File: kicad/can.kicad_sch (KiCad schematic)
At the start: 23 parts, among them CN10 KF2EDGR-2.54-3P, J4 Header-Male-2.54_2x2, U18 ADM3057EBRWZ-RL

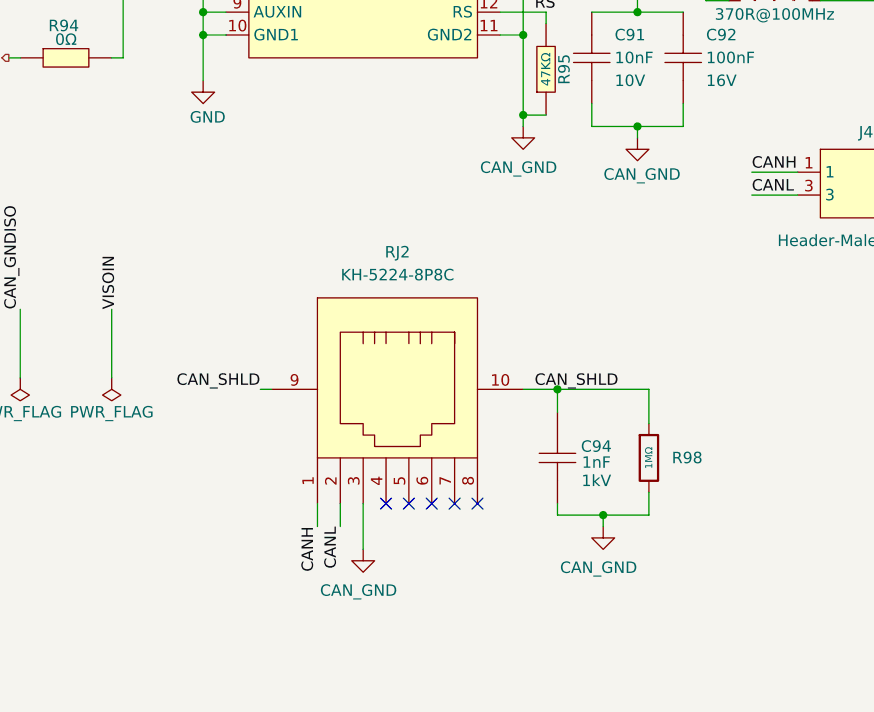
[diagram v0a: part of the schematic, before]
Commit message: Updates
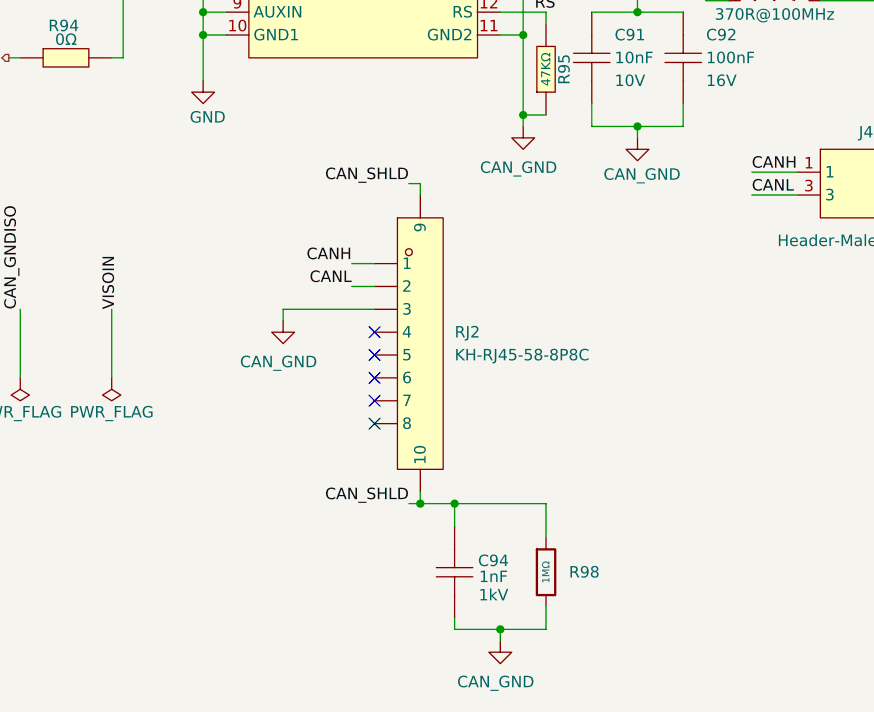
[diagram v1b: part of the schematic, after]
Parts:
- removed RJ2: KH-5224-8P8C, MyParts:RJ45-KH-5224-8P8C, symbol MyParts:KH-5224-8P8C
- added RJ2: KH-RJ45-58-8P8C, MyParts:RJ45-TH_KH-RJ45-58-8P8C, symbol MyParts:KH-RJ45-58-8P8C
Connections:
- net CANH: now also RJ2.1
- net CANL: now also RJ2.2
- net CAN_GND: now also RJ2.3
- net CAN_SHLD: now also RJ2.10, RJ2.9
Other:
- moved on the sheet: C94, R98

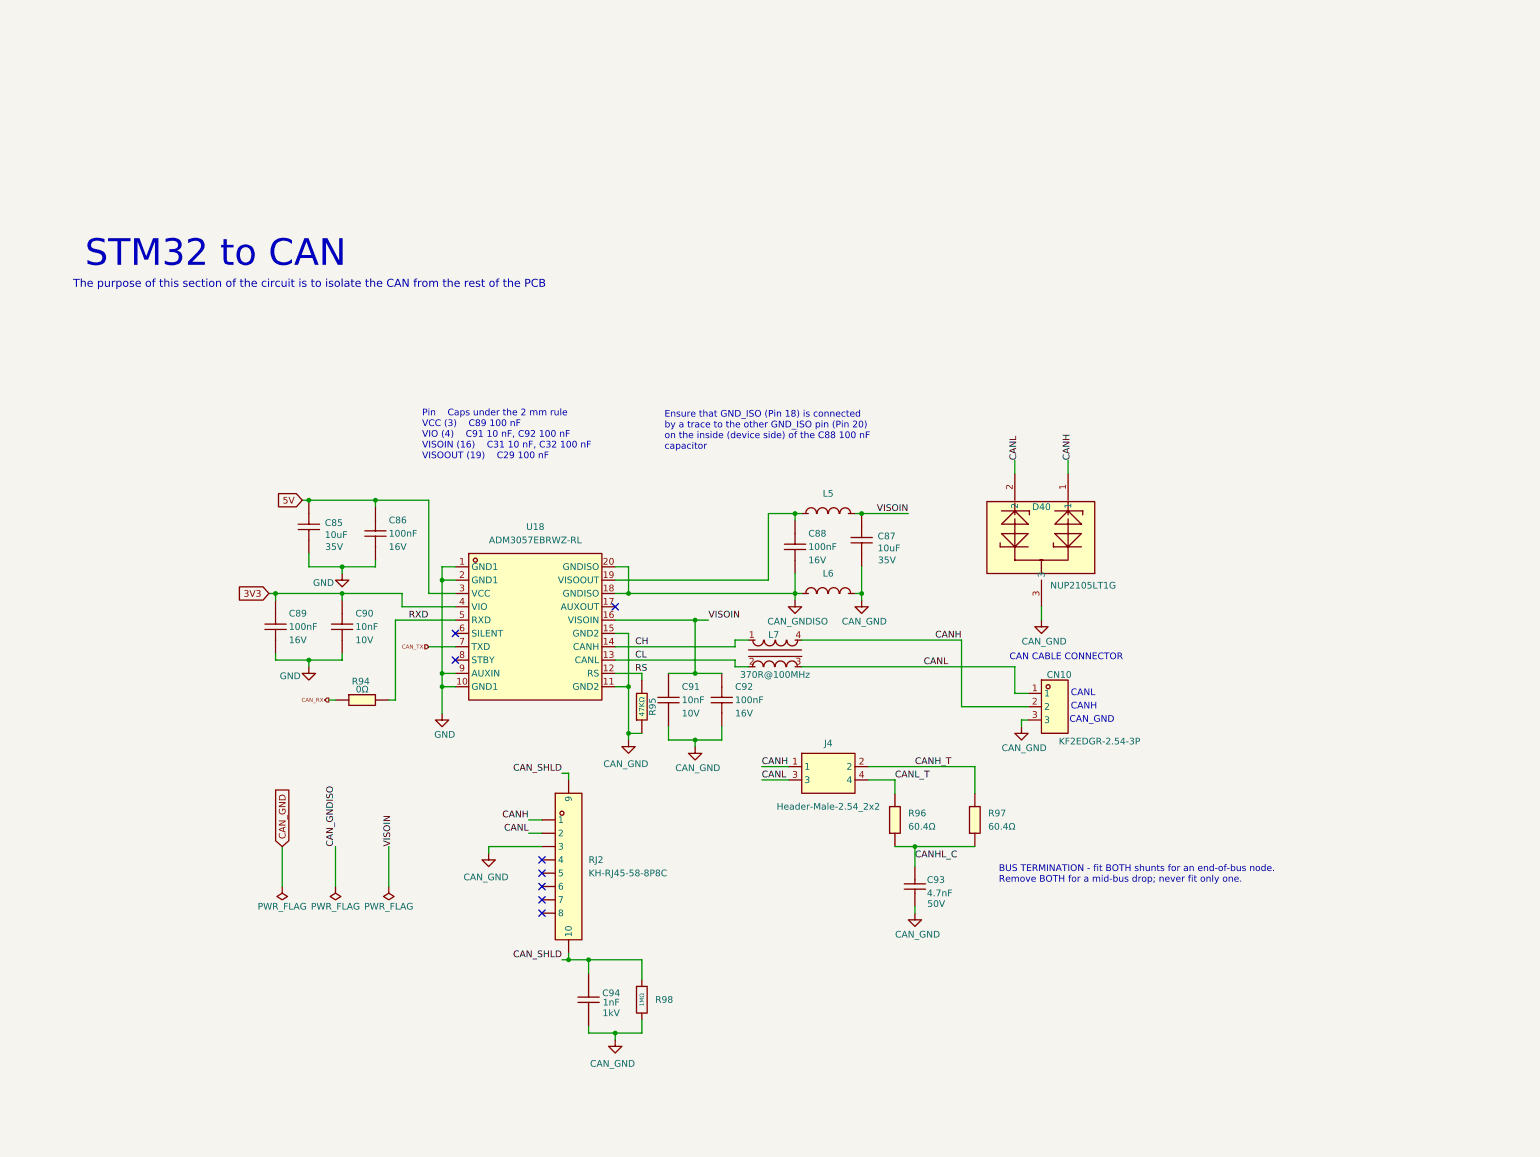
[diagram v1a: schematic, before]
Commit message: Before removing CAN 24V
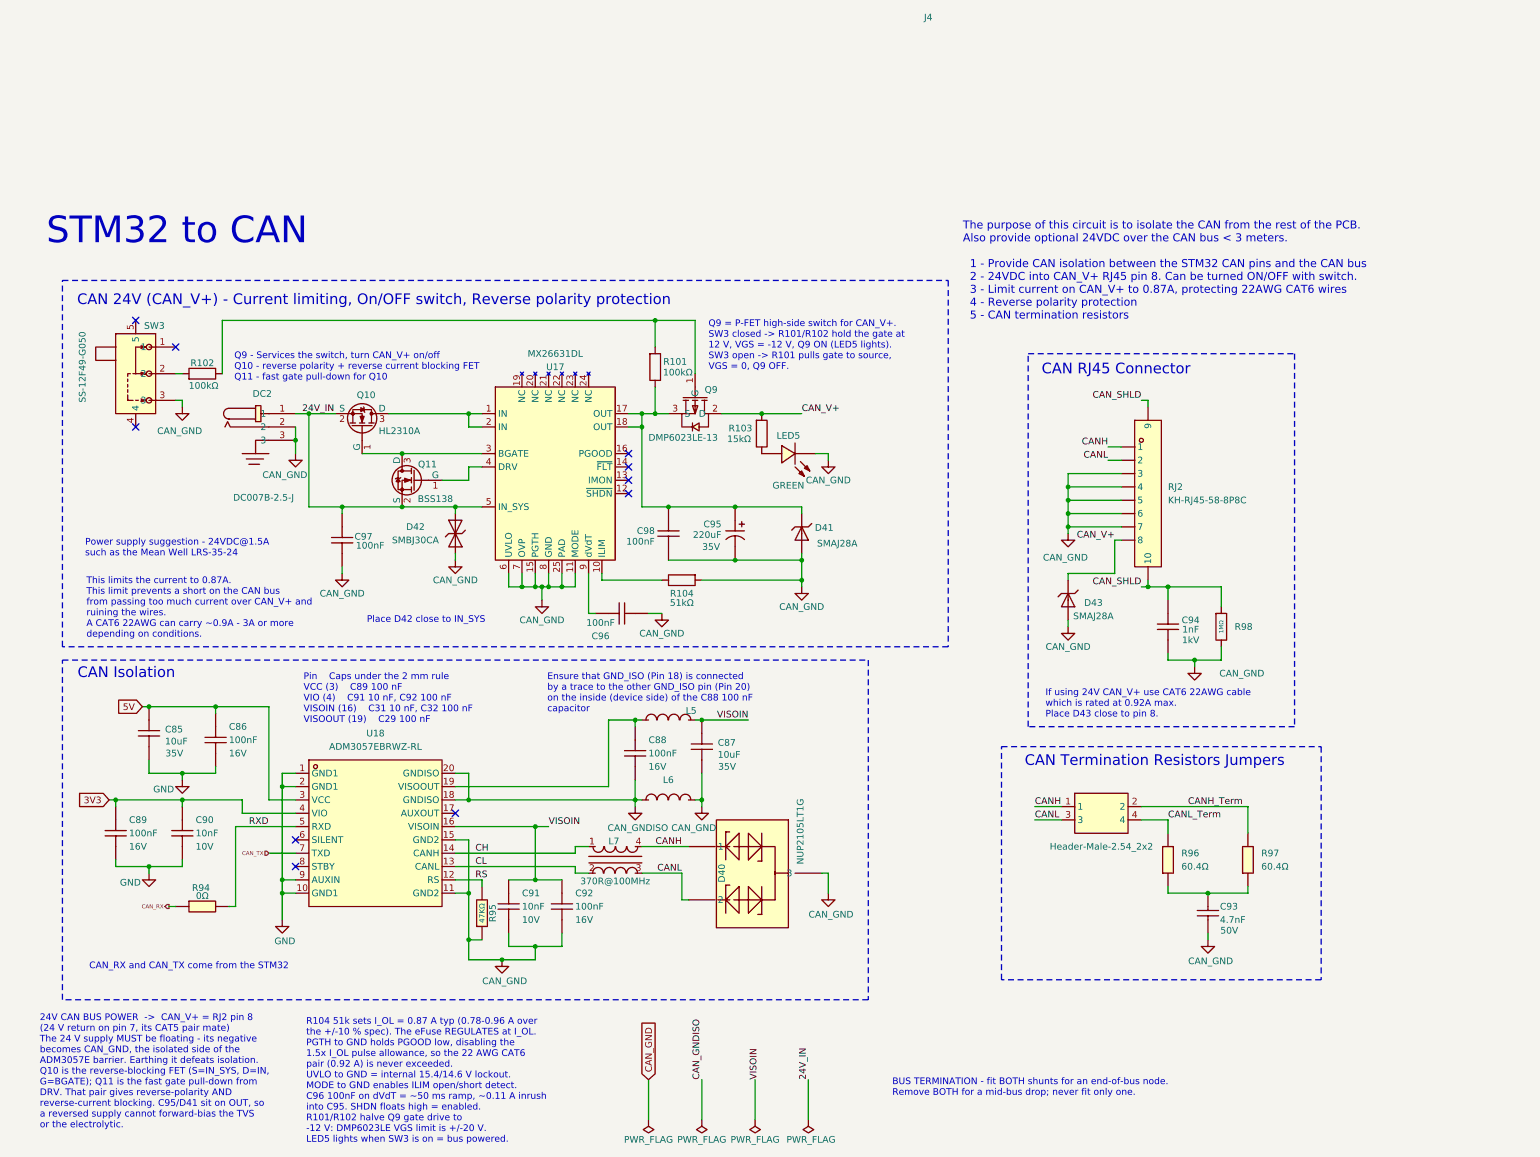
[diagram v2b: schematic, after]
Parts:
- removed CN10: KF2EDGR-2.54-3P, MyParts:CONN-TH_3P-P2.54_KF2EDGR-2.54-3P, symbol MyParts:KF2EDGR-2.54-3P
- added C95: 220uF, MyParts:CAP-SMD_BD6.3-L6.6-W6.6-FD, symbol MyParts:JVJ35V220M6X8
- added C96, C97, C98: 100nF, MyParts:C0402, symbol MyParts:CL05B104KO5NNNC
- added D41, D43: SMAJ28A, PCM_JLCPCB:D_SMA, symbol PCM_JLCPCB-Diodes:TVS-Uni,SMAJ28A
- added D42: SMBJ30CA, PCM_JLCPCB:D_SMB, symbol PCM_JLCPCB-Diodes:TVS-Bi,SMBJ30CA
- added DC2: DC007B-2.5-J, MyParts:DC-IN-TH_HX-DC007B-2.5, symbol MyParts:DC007B-2.5-J
- added LED5: GREEN, MyParts:LED0805-R-RD, symbol MyParts:0805G
- added Q10: HL2310A, PCM_JLCPCB:Q_SOT-23, symbol PCM_JLCPCB-Transistors:NMOS,HL2310A
- added Q11: BSS138, PCM_JLCPCB:Q_SOT-23, symbol PCM_JLCPCB-Transistors:NMOS,BSS138
- added Q9: DMP6023LE-13, Package_TO_SOT_SMD:SOT-223-3_TabPin2, symbol MyParts:DMP6023LE-13
- added R101, R102: 100kΩ, PCM_JLCPCB:R_0603, symbol PCM_JLCPCB-Resistors:0603,100kΩ
- added R103: 15kΩ, PCM_JLCPCB:R_0603, symbol PCM_JLCPCB-Resistors:0603,15kΩ
- added R104: 51kΩ, PCM_JLCPCB:R_0603, symbol PCM_JLCPCB-Resistors:0603,51kΩ
- added SW3: SS-12F49-G050, MyParts:SW-TH_SS-12F45-GXXX, symbol MyParts:SS-12F49-G050
- added U17: MX26631DL, Package_DFN_QFN:QFN-24-1EP_4x4mm_P0.5mm_EP2.7x2.7mm_ThermalVias, symbol MyParts:MX26631DL
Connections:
- net CAN_GND: now also RJ2.4, RJ2.5, RJ2.6, RJ2.7, C95.2, C96.2, C97.1, C98.1, D41.2, D42.2, D43.2, DC2.2, DC2.3, LED5.2 (K), R104.1, SW3.3, U17.11 (MODE), U17.15 (PGTH), U17.25 (PAD), U17.6 (UVLO), U17.7 (OVP), U17.8 (GND)
- net CAN_V+: now reaches RJ2.8
- net CAN_V+: now also D43.1, Q9.2 (D), R103.1
- net CANHL_C: no longer names the net of C93.1, R96.1, R97.1
- net CANH_T renamed CANH_Term
- net CANL_T renamed CANL_Term
- new net: Q10.3 (D), U17.1 (IN), U17.2 (IN)
- new net: R104.2, U17.10 (ILIM)
- new net: C95.1, C98.2, D41.1, Q9.3 (S), R101.2, U17.17 (OUT), U17.18 (OUT)
- new net: Q10.1 (G), Q11.3 (D), U17.3 (BGATE)
- new net: Q11.1 (G), U17.4 (DRV)
- new net: C96.1, U17.9 (dVdT)
- new net: Q9.1 (G), R101.1, R102.2
- new net: R102.1, SW3.2
- new net: LED5.1 (A), R103.2
- new net 24V_IN: C97.2, D42.1, DC2.1, Q10.2 (S), Q11.2 (S), U17.5 (IN_SYS)
- no-connect marks 8 -> 10
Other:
- note added: "24V CAN BUS POWER -> CAN_V+ = RJ2 pin 8 (24 V return on pin 7, its CAT5 pair mate) The 24 V supply MUST be floating - its negative becomes CAN_GND, the isolated side of the ADM3057E barrier. Earthing it defeats isolation. Q10 is the reverse-blocking FET (S=IN_SYS, D=IN, G=BGATE); Q11 is the fast gate pull-down from DRV. That pair gives reverse-polarity AND reverse-current blocking. C95/D41 sit on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"
- note added: "CAN 24V (CAN_V+) - Current limiting, On/OFF switch, Reverse polarity protection"
- note added: "CAN Isolation"
- note added: "CAN RJ45 Connector"
- note added: "CAN Termination Resistors Jumpers"
- note added: "CAN_RX and CAN_TX come from the STM32"
- note added: "If using 24V CAN_V+ use CAT6 22AWG cable which is rated at 0.92A max. Place D43 close to pin 8."
- note added: "Place D42 close to IN_SYS"
- note added: "Power supply suggestion - 24VDC@1.5A such as the Mean Well LRS-35-24"
- note added: "Q9 - Services the switch, turn CAN_V+ on/off Q10 - reverse polarity + reverse current blocking FET Q11 - fast gate pull-down for Q10"
- note added: "Q9 = P-FET high-side switch for CAN_V+. SW3 closed -> R101/R102 hold the gate at 12 V, VGS = -12 V, Q9 ON (LED5 lights). SW3 open -> R101 pulls gate to source, VGS = 0, Q9 OFF."
- note added: "R104 51k sets I_OL = 0.87 A typ (0.78-0.96 A over the +/-10 % spec). The eFuse REGULATES at I_OL. PGTH to GND holds PGOOD low, disabling the 1.5x I_OL pulse allowance, so the 22 AWG CAT6 pair (0.92 A) is never exceeded. UVLO to GND = internal 15.4/14.6 V lockout. MODE to GND enables ILIM open/short detect. C96 100nF on dVdT = ~50 ms ramp, ~0.11 A inrush into C95. SHDN floats high = enabled. R101/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"
- note added: "The purpose of this circuit is to isolate the CAN from the rest of the PCB. Also provide optional 24VDC over the CAN bus < 3 meters. 1 - Provide CAN isolation between the STM32 CAN pins and the CAN bus 2 - 24VDC into CAN_V+ RJ45 pin 8. Can be turned ON/OFF with switch. 3 - Limit current on CAN_V+ to 0.87A, protecting 22AWG CAT6 wires 4 - Reverse polarity protection 5 - CAN termination resistors"
- note added: "This limits the current to 0.87A. This limit prevents a short on the CAN bus from passing too much current over CAN_V+ and ruining the wires. A CAT6 22AWG can carry ~0.9A - 3A or more depending on conditions."
- note removed: "CAN CABLE CONNECTOR"
- note removed: "CANH"
- note removed: "CANL"
- note removed: "CAN_GND"
- note removed: "The purpose of this section of the circuit is to isolate the CAN from the rest of the PCB"
- moved on the sheet: C85, C86, C87, C88, C89, C90, C91, C92, C93, C94, J4, L5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

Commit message: Refinements
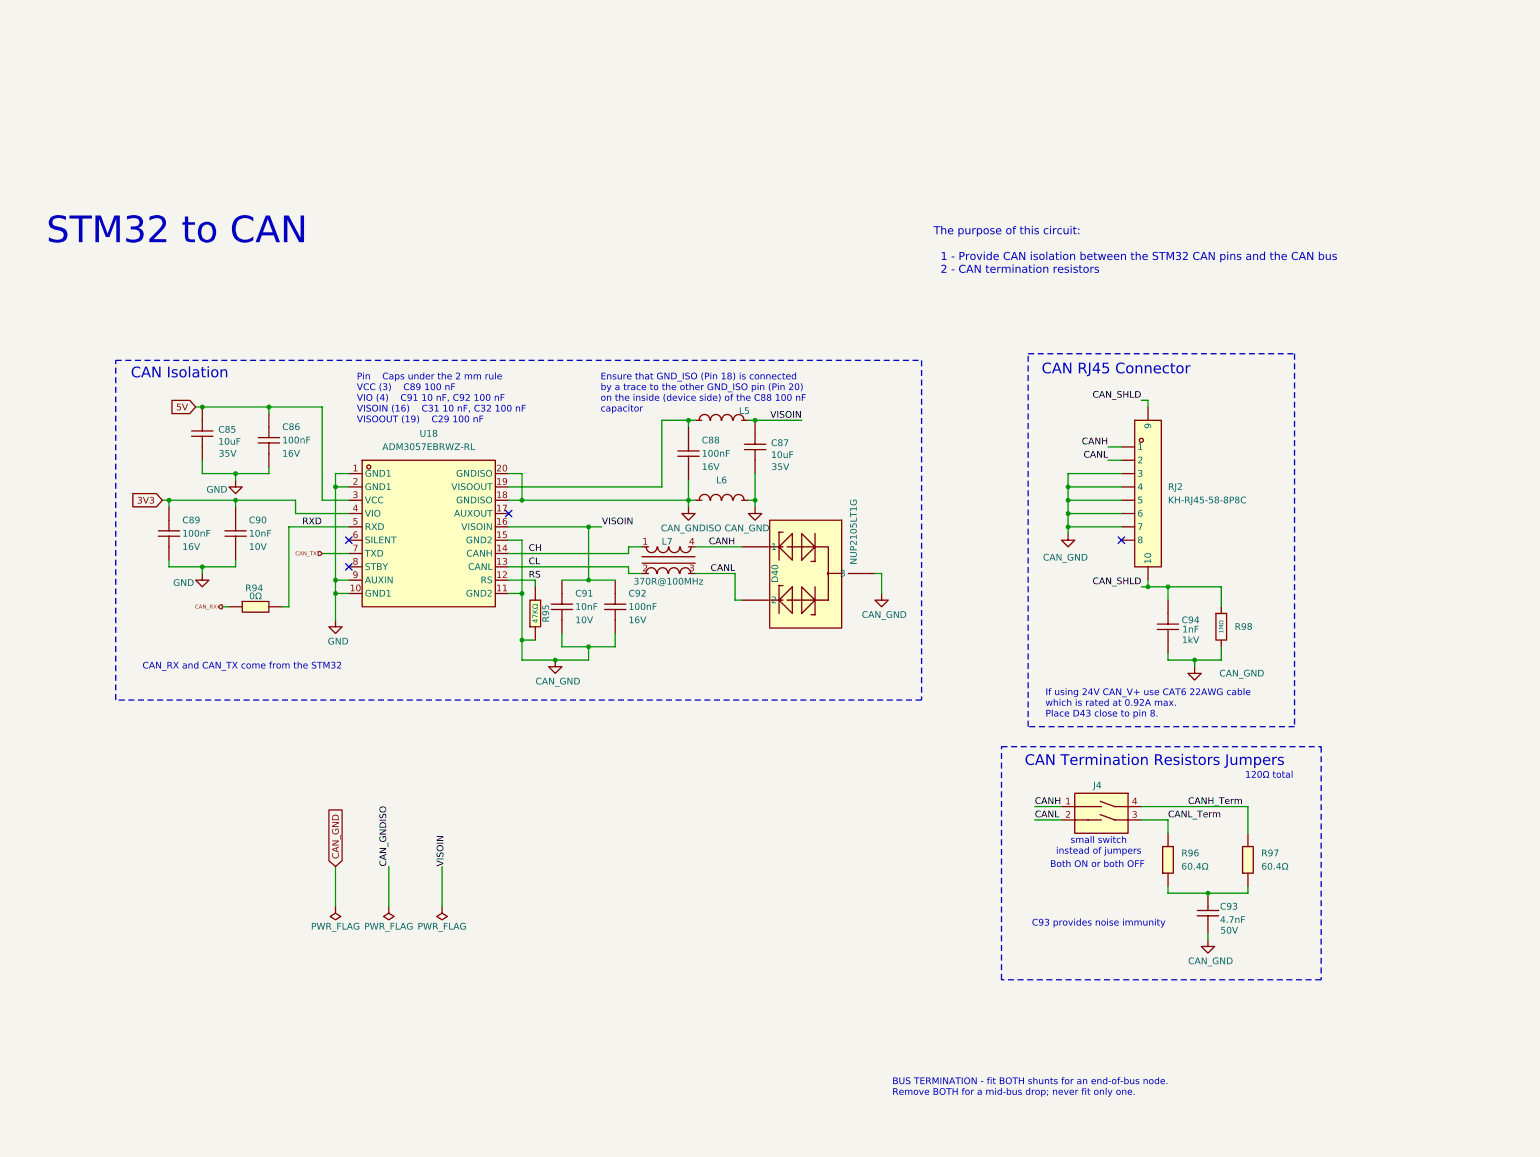
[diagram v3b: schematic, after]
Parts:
- removed C95: 220uF, MyParts:CAP-SMD_BD6.3-L6.6-W6.6-FD, symbol MyParts:JVJ35V220M6X8
- removed C96, C97, C98: 100nF, MyParts:C0402, symbol MyParts:CL05B104KO5NNNC
- removed D41, D43: SMAJ28A, PCM_JLCPCB:D_SMA, symbol PCM_JLCPCB-Diodes:TVS-Uni,SMAJ28A
- removed D42: SMBJ30CA, PCM_JLCPCB:D_SMB, symbol PCM_JLCPCB-Diodes:TVS-Bi,SMBJ30CA
- removed DC2: DC007B-2.5-J, MyParts:DC-IN-TH_HX-DC007B-2.5, symbol MyParts:DC007B-2.5-J
- removed J4: Header-Male-2.54_2x2, MyParts:HDR-TH_4P-P2.54-V-M-R2-C2-S2.54-1, symbol MyParts:Header-Male-2.54_2x2
- removed LED5: GREEN, MyParts:LED0805-R-RD, symbol MyParts:0805G
- removed Q10: HL2310A, PCM_JLCPCB:Q_SOT-23, symbol PCM_JLCPCB-Transistors:NMOS,HL2310A
- removed Q11: BSS138, PCM_JLCPCB:Q_SOT-23, symbol PCM_JLCPCB-Transistors:NMOS,BSS138
- removed Q9: DMP6023LE-13, Package_TO_SOT_SMD:SOT-223-3_TabPin2, symbol MyParts:DMP6023LE-13
- removed R101, R102: 100kΩ, PCM_JLCPCB:R_0603, symbol PCM_JLCPCB-Resistors:0603,100kΩ
- removed R103: 15kΩ, PCM_JLCPCB:R_0603, symbol PCM_JLCPCB-Resistors:0603,15kΩ
- removed R104: 51kΩ, PCM_JLCPCB:R_0603, symbol PCM_JLCPCB-Resistors:0603,51kΩ
- removed SW3: SS-12F49-G050, MyParts:SW-TH_SS-12F45-GXXX, symbol MyParts:SS-12F49-G050
- removed U17: MX26631DL, Package_DFN_QFN:QFN-24-1EP_4x4mm_P0.5mm_EP2.7x2.7mm_ThermalVias, symbol MyParts:MX26631DL
- added J4: DSHP02TSGER, MyParts:SW-SMD_DSHP02TSGER, symbol MyParts:DSHP02TSGER
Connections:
- net CANH: now also J4.1
- net CANH_Term: now also J4.4
- net CANL: now also J4.2
- net CANL_Term: now also J4.3
- net CAN_V+: no longer names the net of RJ2.8
- no-connect marks 10 -> 4
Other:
- note added: "120Ω total"
- note added: "Both ON or both OFF"
- note added: "C93 provides noise immunity"
- note added: "The purpose of this circuit: 1 - Provide CAN isolation between the STM32 CAN pins and the CAN bus 2 - CAN termination resistors"
- note added: "small switch instead of jumpers"
- note removed: "24V CAN BUS POWER -> CAN_V+ = RJ2 pin 8 (24 V return on pin 7, its CAT5 pair mate) The 24 V supply MUST be floating - its negative becomes CAN_GND, the isolated side of the ADM3057E barrier. Earthing it defeats isolation. Q10 is the reverse-blocking FET (S=IN_SYS, D=IN, G=BGATE); Q11 is the fast gate pull-down from DRV. That pair gives reverse-polarity AND reverse-current blocking. C95/D41 sit on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"
- note removed: "CAN 24V (CAN_V+) - Current limiting, On/OFF switch, Reverse polarity protection"
- note removed: "Place D42 close to IN_SYS"
- note removed: "Power supply suggestion - 24VDC@1.5A such as the Mean Well LRS-35-24"
- note removed: "Q9 - Services the switch, turn CAN_V+ on/off Q10 - reverse polarity + reverse current blocking FET Q11 - fast gate pull-down for Q10"
- note removed: "Q9 = P-FET high-side switch for CAN_V+. SW3 closed -> R101/R102 hold the gate at 12 V, VGS = -12 V, Q9 ON (LED5 lights). SW3 open -> R101 pulls gate to source, VGS = 0, Q9 OFF."
- note removed: "R104 51k sets I_OL = 0.87 A typ (0.78-0.96 A over the +/-10 % spec). The eFuse REGULATES at I_OL. PGTH to GND holds PGOOD low, disabling the 1.5x I_OL pulse allowance, so the 22 AWG CAT6 pair (0.92 A) is never exceeded. UVLO to GND = internal 15.4/14.6 V lockout. MODE to GND enables ILIM open/short detect. C96 100nF on dVdT = ~50 ms ramp, ~0.11 A inrush into C95. SHDN floats high = enabled. R101/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"
- note removed: "The purpose of this circuit is to isolate the CAN from the rest of the PCB. Also provide optional 24VDC over the CAN bus < 3 meters. 1 - Provide CAN isolation between the STM32 CAN pins and the CAN bus 2 - 24VDC into CAN_V+ RJ45 pin 8. Can be turned ON/OFF with switch. 3 - Limit current on CAN_V+ to 0.87A, protecting 22AWG CAT6 wires 4 - Reverse polarity protection 5 - CAN termination resistors"
- note removed: "This limits the current to 0.87A. This limit prevents a short on the CAN bus from passing too much current over CAN_V+ and ruining the wires. A CAT6 22AWG can carry ~0.9A - 3A or more depending on conditions."
- moved on the sheet: C85, C86, C87, C88, C89, C90, C91, C92, D40, L5, L6, L7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
